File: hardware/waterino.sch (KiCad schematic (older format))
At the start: 47 parts, among them CON1 POWER, P1 PUMP, P2 PLANT, P3 UART, P4 CONN_02X06, P5 CONN_01X04, P6 CONN_01X03, SW1 RESET, U1 LM7805CT, U2 MIC94090, U3 ATMEGA168-20AU

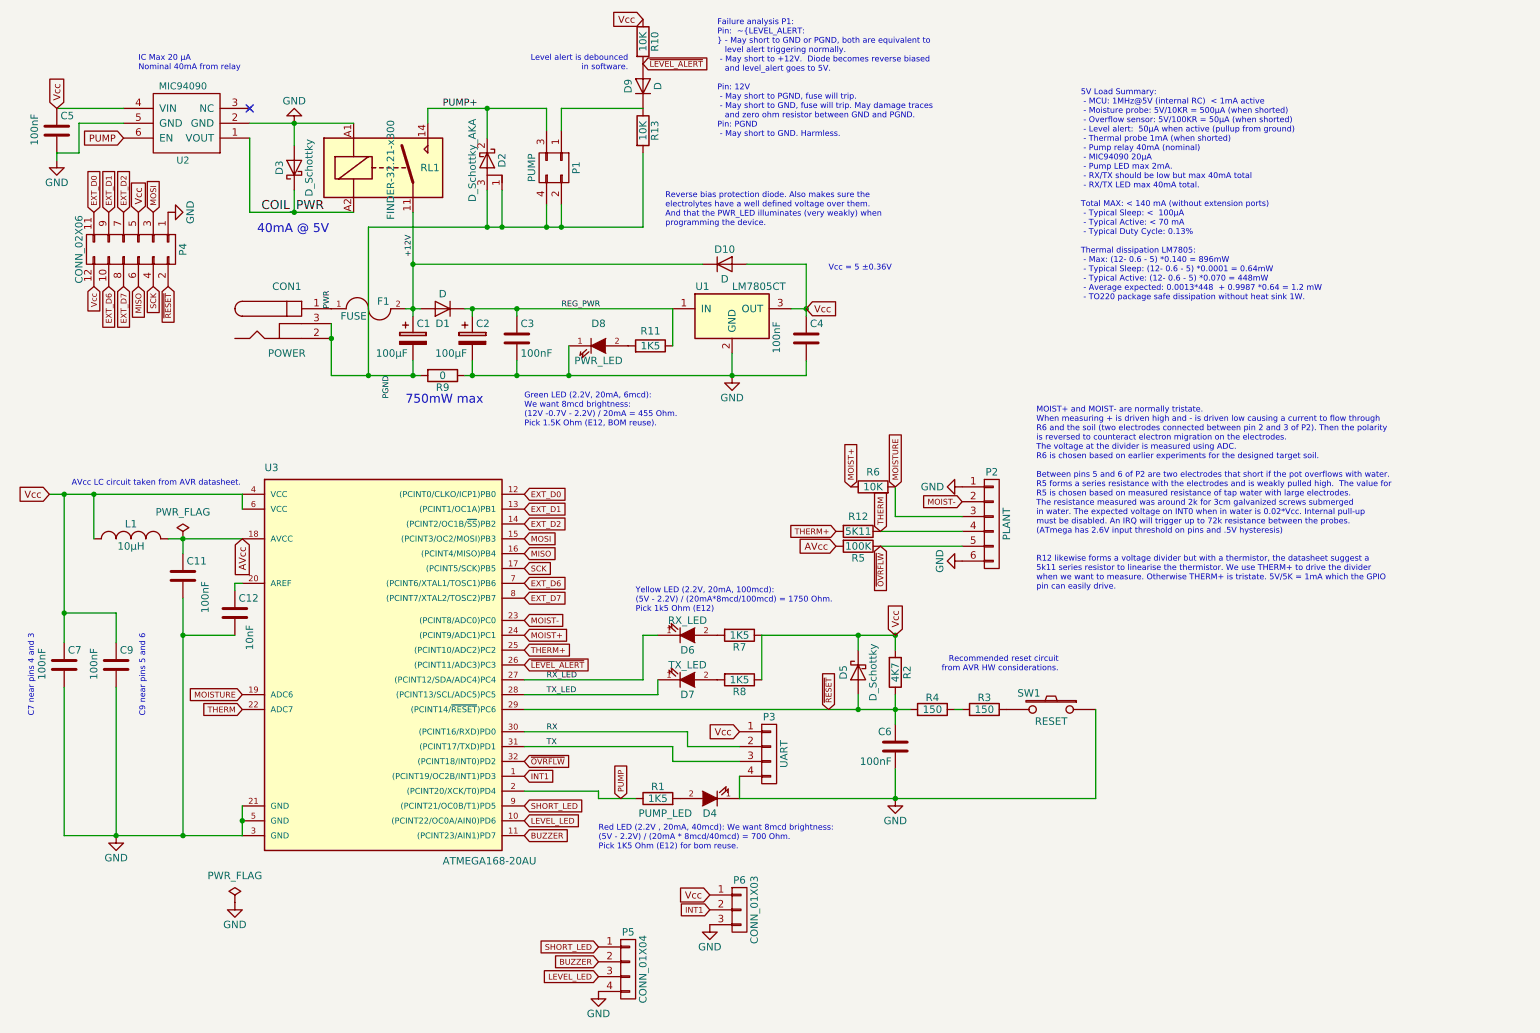
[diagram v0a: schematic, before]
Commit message: Adding schematic for the probe.
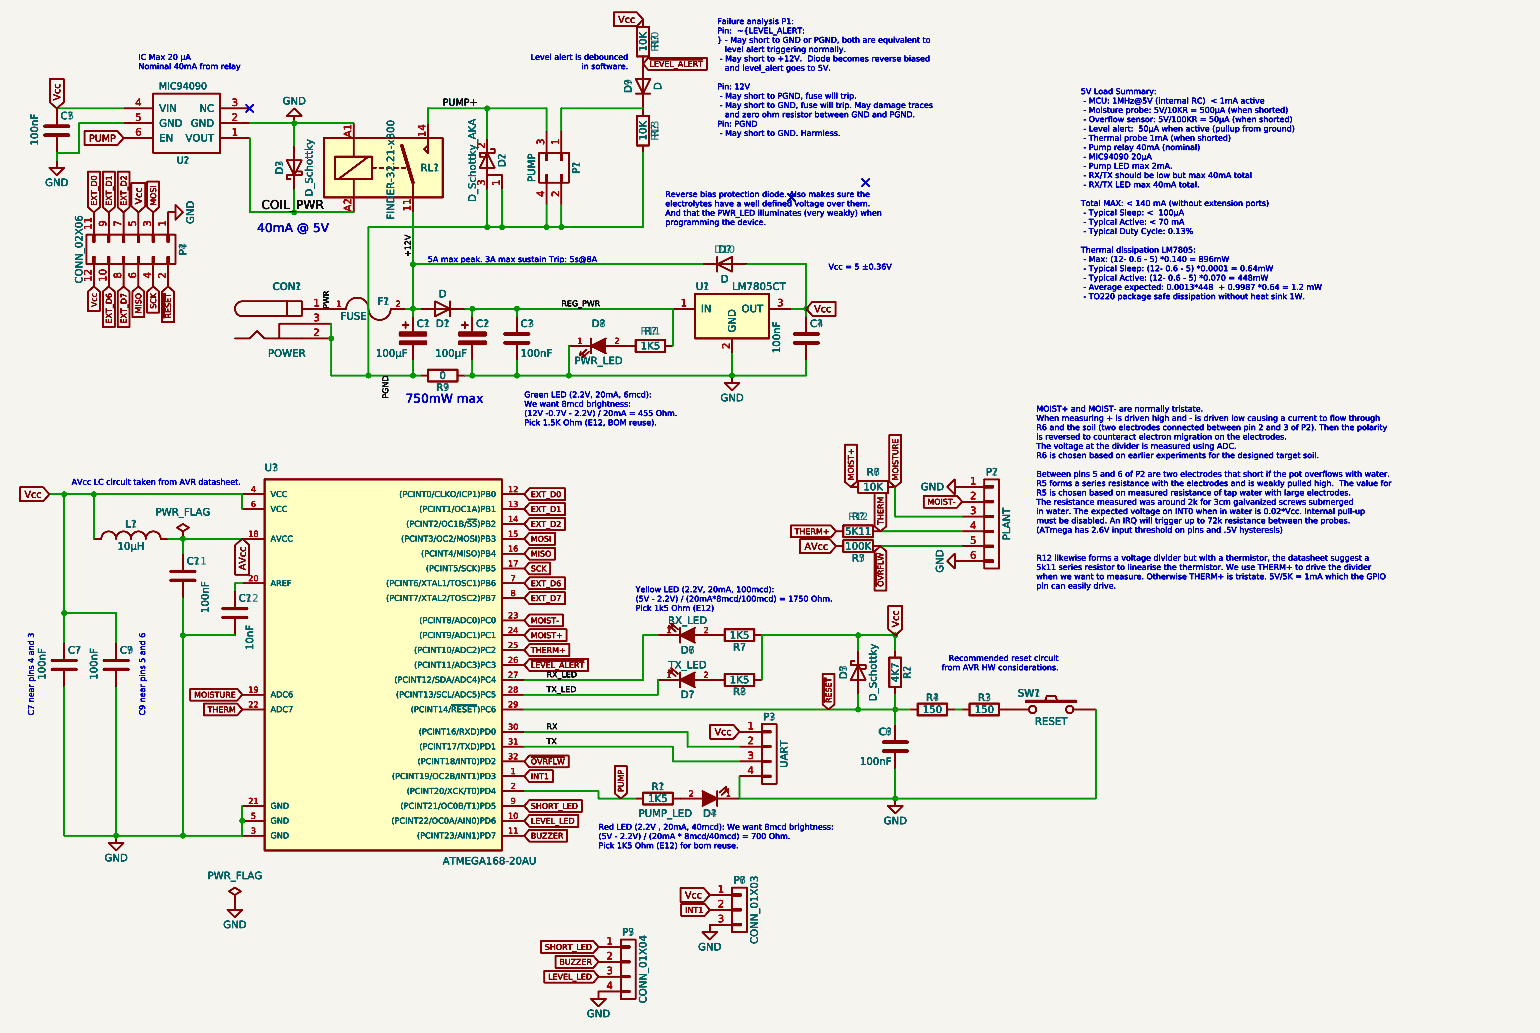
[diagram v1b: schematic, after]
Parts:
- added C? (x14): 100nF, Capacitors_SMD:C_0603, symbol C
- added C? (x4): 100µF, Capacitors_SMD:CP_Elec_6.3x7.7, symbol CP
- added C? (x2): 10nF, Capacitors_SMD:C_0603, symbol C
- added CON? (x2): POWER, Connectors:BARREL_JACK, symbol BARREL_JACK
- added D? (x2): PWR_LED, LEDs:LED_0603, symbol LED-RESCUE-waterino
- added D? (x2): PUMP_LED, LEDs:LED_0603, symbol LED-RESCUE-waterino
- added D? (x2): TX_LED, LEDs:LED_0603, symbol LED-RESCUE-waterino
- added D? (x2): RX_LED, LEDs:LED_0603, symbol LED-RESCUE-waterino
- added D? (x4): D, Diodes_THT:D_DO-41_SOD81_P7.62mm_Horizontal, symbol D
- added D? (x4): D_Schottky, Diodes_SMD:D_SOD-123, symbol D_Schottky
- added D? (x2): D_Schottky_AKA, TO_SOT_Packages_SMD:TO-252-2_Rectifier, symbol D_Schottky_AKA
- added D? (x2): D, Diodes_ThroughHole:D_DO-41_SOD81_P7.62mm_Horizontal, symbol D
- added F? (x2): FUSE, Fuse_Holders_and_Fuses:Fuse_SMD2920, symbol FUSE
- added L? (x2): 10µH, Inductors_THT:L_Axial_L7.0mm_D3.3mm_P10.16mm_Horizontal_Fastron_MICC, symbol INDUCTOR_SMALL
- added P? (x2): UART, Pin_Headers:Pin_Header_Straight_1x04_Pitch2.54mm, symbol CONN_01X04
- added P? (x2): PUMP, Connectors_Molex:Molex_Microfit3_Header_02x02_Angled_43045-040x, symbol CONN_02X02
- added P? (x2): PLANT, Connectors_JST:JST_PH_S6B-PH-K_06x2.00mm_Angled, symbol CONN_01X06
- added P? (x2): CONN_01X04, Pin_Headers:Pin_Header_Straight_2x02_Pitch2.54mm, symbol CONN_01X04
- added P? (x2): CONN_01X03, Pin_Headers:Pin_Header_Straight_1x03_Pitch2.54mm, symbol CONN_01X03
- added P? (x2): CONN_02X06, Pin_Headers:Pin_Header_Straight_2x06_Pitch2.54mm, symbol CONN_02X06
- added R? (x6): 10K, Resistors_SMD:R_0603, symbol R
- added R? (x2): 100K, Resistors_SMD:R_0603, symbol R
- added R? (x8): 1K5, Resistors_SMD:R_0603, symbol R
- added R? (x2): 0, Resistors_SMD:R_2010, symbol R
- added R? (x2): 4K7, Resistors_SMD:R_0603, symbol R
- added R? (x4): 150, Resistors_SMD:R_0603, symbol R
- added R? (x2): 5K11, Resistors_SMD:R_0603, symbol R
- added RL? (x2): FINDER-32.21-x300, Relays_THT:Relay_SPST_Finder_32.21-x300, symbol FINDER-32.21-x300
- added SW? (x2): RESET, Buttons_Switches_THT:SW_PUSH_6mm, symbol SW_PUSH
- added U? (x2): MIC94090, TO_SOT_Packages_SMD:SOT-363_SC-70-6_Handsoldering, symbol MIC94090
- added U? (x2): ATMEGA168-20AU, Housings_QFP:TQFP-32_7x7mm_Pitch0.8mm, symbol ATMEGA168-20AU
- added U? (x2): LM7805CT, Power_Integrations:TO-220, symbol LM7805CT
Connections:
- net +12V: now also C?.1, C?.1, D?.1 (K), D?.1 (K), D?.2 (A), D?.2 (A), F?.2, F?.2, RL?.11, RL?.11
- net AVcc: now also C?.1, C?.1, L?.2, L?.2, R?.2, R?.2, U?.18 (AVCC), U?.18 (AVCC)
- net BUZZER: now also P?.2 (P2), P?.2 (P2), U?.11 ((PCINT23/AIN1)PD7), U?.11 ((PCINT23/AIN1)PD7)
- net COIL_PWR: now also D?.1 (K), D?.1 (K), RL?.A2, RL?.A2, U?.1 (VOUT), U?.1 (VOUT)
- net EXT_D0: now also P?.11 (P11), P?.11 (P11), U?.12 ((PCINT0/CLKO/ICP1)PB0), U?.12 ((PCINT0/CLKO/ICP1)PB0)
- net EXT_D1: now also P?.9 (P9), P?.9 (P9), U?.13 ((PCINT1/OC1A)PB1), U?.13 ((PCINT1/OC1A)PB1)
- net EXT_D2: now also P?.7 (P7), P?.7 (P7), U?.14 ((PCINT2/OC1B/~SS~)PB2), U?.14 ((PCINT2/OC1B/~SS~)PB2)
- net EXT_D6: now also P?.10 (P10), P?.10 (P10), U?.7 ((PCINT6/XTAL1/TOSC1)PB6), U?.7 ((PCINT6/XTAL1/TOSC1)PB6)
- net EXT_D7: now also P?.8 (P8), P?.8 (P8), U?.8 ((PCINT7/XTAL2/TOSC2)PB7), U?.8 ((PCINT7/XTAL2/TOSC2)PB7)
- net GND: now also C?.2, C?.2, C?.2, C?.2, C?.2, C?.2, C?.2, C?.2, C?.2, C?.2, C?.2, C?.2, C?.2, C?.2, C?.2, C?.2, C?.2, C?.2, D?.1 (K), D?.1 (K), D?.1 (K), D?.1 (K), D?.2 (A), D?.2 (A), P?.1 (P1), P?.1 (P1), P?.1 (P1), P?.1 (P1), P?.3 (P3), P?.3 (P3), P?.4 (P4), P?.4 (P4), P?.4 (P4), P?.4 (P4), P?.6 (P6), P?.6 (P6), R?.1, R?.1, RL?.A1, RL?.A1, SW?.1, SW?.1, U?.2 (GND), U?.2 (GND), U?.2 (GND), U?.2 (GND), U?.21 (GND), U?.21 (GND), U?.3 (GND), U?.3 (GND), U?.5 (GND), U?.5 (GND), U?.5 (GND), U?.5 (GND)
- net INT1: now also P?.2 (P2), P?.2 (P2), U?.1 ((PCINT19/OC2B/INT1)PD3), U?.1 ((PCINT19/OC2B/INT1)PD3)
- net LEVEL_LED: now also P?.3 (P3), P?.3 (P3), U?.10 ((PCINT22/OC0A/AIN0)PD6), U?.10 ((PCINT22/OC0A/AIN0)PD6)
- net MISO: now also P?.6 (P6), P?.6 (P6), U?.16 ((PCINT4/MISO)PB4), U?.16 ((PCINT4/MISO)PB4)
- net MOIST+: now also R?.1, R?.1, U?.24 ((PCINT9/ADC1)PC1), U?.24 ((PCINT9/ADC1)PC1)
- net MOIST-: now also P?.2 (P2), P?.2 (P2), U?.23 ((PCINT8/ADC0)PC0), U?.23 ((PCINT8/ADC0)PC0)
- net MOISTURE: now also P?.3 (P3), P?.3 (P3), R?.2, R?.2, U?.19 (ADC6), U?.19 (ADC6)
- net MOSI: now also P?.3 (P3), P?.3 (P3), U?.15 ((PCINT3/OC2/MOSI)PB3), U?.15 ((PCINT3/OC2/MOSI)PB3)
- net PGND: now also C?.2, C?.2, CON?.2, CON?.2, CON?.3, CON?.3, D?.1 (A), D?.1 (A), D?.3 (A), D?.3 (A), P?.2 (P2), P?.2 (P2), P?.4 (P4), P?.4 (P4), R?.2, R?.2, R?.2, R?.2
- net PUMP: now also R?.1, R?.1, U?.2 ((PCINT20/XCK/T0)PD4), U?.2 ((PCINT20/XCK/T0)PD4), U?.6 (EN), U?.6 (EN)
- net PUMP+: now also D?.2 (K), D?.2 (K), P?.3 (P3), P?.3 (P3), RL?.14, RL?.14
- net PWR: now also CON?.1, CON?.1, F?.1, F?.1
- net REG_PWR: now also C?.1, C?.1, C?.1, C?.1, D?.1 (K), D?.1 (K), R?.1, R?.1, U?.1 (IN), U?.1 (IN)
- net RX: now also P?.2 (P2), P?.2 (P2), U?.30 ((PCINT16/RXD)PD0), U?.30 ((PCINT16/RXD)PD0)
- net RX_LED: now also D?.1 (K), D?.1 (K), U?.27 ((PCINT12/SDA/ADC4)PC4), U?.27 ((PCINT12/SDA/ADC4)PC4)
- net SCK: now also P?.4 (P4), P?.4 (P4), U?.17 ((PCINT5/SCK)PB5), U?.17 ((PCINT5/SCK)PB5)
- net SHORT_LED: now also P?.1 (P1), P?.1 (P1), U?.9 ((PCINT21/OC0B/T1)PD5), U?.9 ((PCINT21/OC0B/T1)PD5)
- net THERM: now also P?.4 (P4), P?.4 (P4), R?.1, R?.1, U?.22 (ADC7), U?.22 (ADC7)
- net THERM+: now also R?.2, R?.2, U?.25 ((PCINT10/ADC2)PC2), U?.25 ((PCINT10/ADC2)PC2)
- net TX: now also P?.3 (P3), P?.3 (P3), U?.31 ((PCINT17/TXD)PD1), U?.31 ((PCINT17/TXD)PD1)
- net TX_LED: now also D?.1 (K), D?.1 (K), U?.28 ((PCINT13/SCL/ADC5)PC5), U?.28 ((PCINT13/SCL/ADC5)PC5)
- net Vcc: now also C?.1, C?.1, C?.1, C?.1, C?.1, C?.1, C?.1, C?.1, D?.1 (K), D?.1 (K), D?.2 (A), D?.2 (A), L?.1, L?.1, P?.1 (P1), P?.1 (P1), P?.1 (P1), P?.1 (P1), P?.12 (P12), P?.12 (P12), P?.5 (P5), P?.5 (P5), R?.1, R?.1, R?.1, R?.1, R?.1, R?.1, R?.2, R?.2, U?.3 (OUT), U?.3 (OUT), U?.4 (VCC), U?.4 (VCC), U?.4 (VIN), U?.4 (VIN), U?.6 (VCC), U?.6 (VCC)
- net ~LEVEL_ALERT: now also D?.2 (A), D?.2 (A), R?.2, R?.2, U?.26 ((PCINT11/ADC3)PC3), U?.26 ((PCINT11/ADC3)PC3)
- net ~OVRFLW: now also P?.5 (P5), P?.5 (P5), R?.1, R?.1, U?.32 ((PCINT18/INT0)PD2), U?.32 ((PCINT18/INT0)PD2)
- net ~RESET: now also C?.1, C?.1, D?.2 (A), D?.2 (A), P?.2 (P2), P?.2 (P2), R?.1, R?.1, R?.2, R?.2, U?.29 ((PCINT14/~RESET~)PC6), U?.29 ((PCINT14/~RESET~)PC6)
- net at U2.3 (NC): now also U?.3 (NC), U?.3 (NC)
- net at D8.2 (A), R11.2: now also D?.2 (A), D?.2 (A), R?.2, R?.2
- net at D4.2 (A), R1.2: now also D?.2 (A), D?.2 (A), R?.2, R?.2
- net at R3.1, SW1.2: now also R?.1, R?.1, SW?.2, SW?.2
- net at D7.2 (A), R8.2: now also D?.2 (A), D?.2 (A), R?.2, R?.2
- net at D6.2 (A), R7.2: now also D?.2 (A), D?.2 (A), R?.2, R?.2
- net at D9.1 (K), P1.1 (P1), R13.1: now also D?.1 (K), D?.1 (K), P?.1 (P1), P?.1 (P1), R?.1, R?.1
- net at R3.2, R4.1: now also R?.1, R?.1, R?.2, R?.2
- net at C12.1, U3.20 (AREF): now also C?.1, C?.1, U?.20 (AREF), U?.20 (AREF)
- no-connect marks 1 -> 9
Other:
- note added: "5A max peak. 3A max sustain Trip: 5s@8A"
